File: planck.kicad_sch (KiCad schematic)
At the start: 53 parts, among them J1 USB_C_Receptacle_USB2.0, K1 KEYSW, K2 KEYSW, K3 KEYSW, K4 KEYSW, SW1 SW_PUSH, U1 ATmega32U4-M, Y1 Crystal_GND24_Small

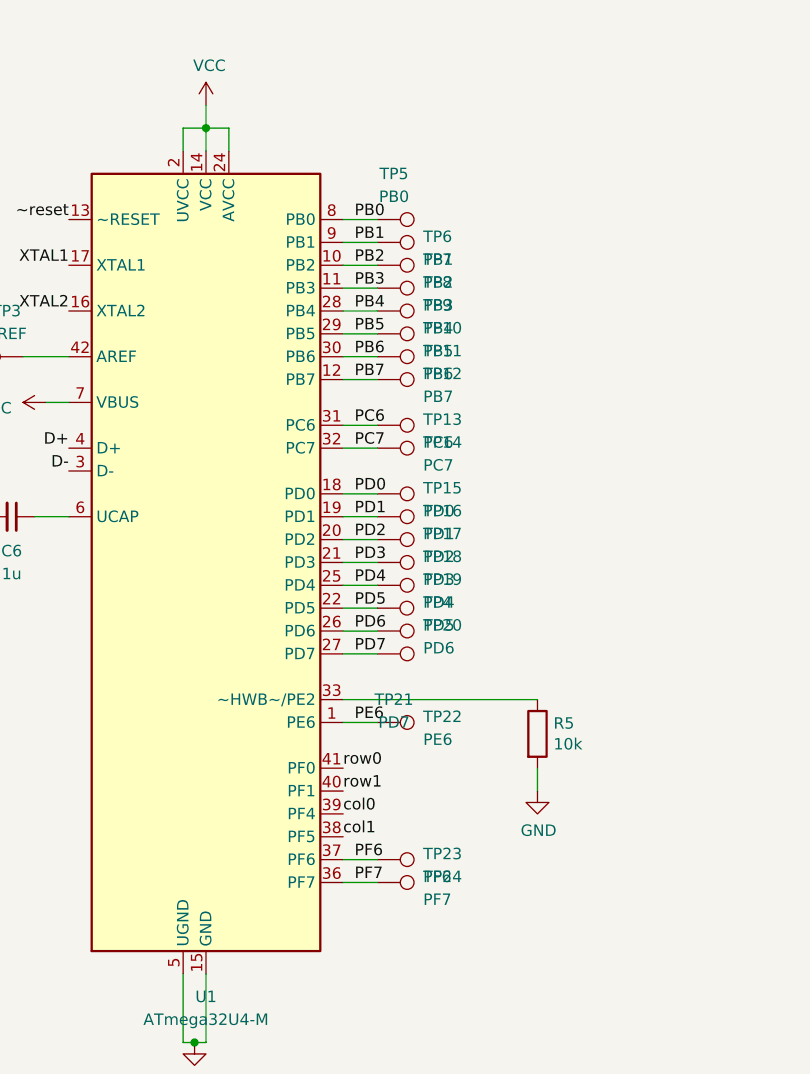
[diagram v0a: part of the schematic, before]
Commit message: finishing it off
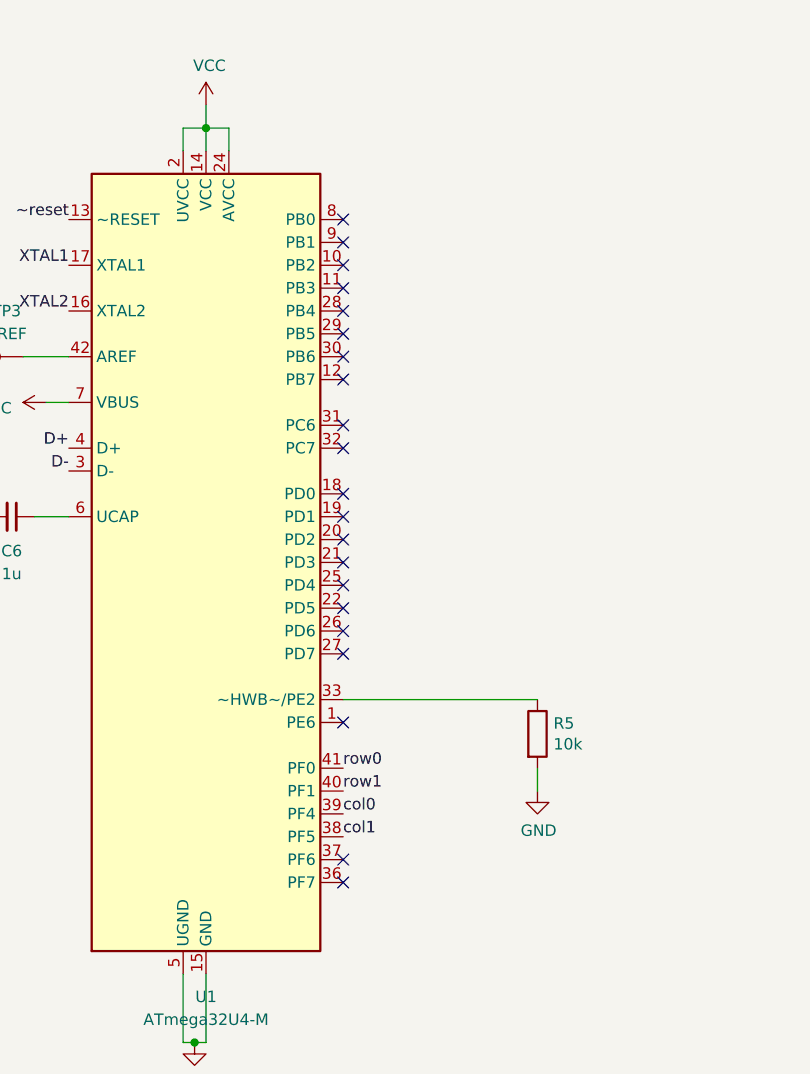
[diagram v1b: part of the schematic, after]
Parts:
- removed TP10: PB5, TestPoint:TestPoint_Pad_D1.0mm, symbol Connector:TestPoint
- removed TP11: PB6, TestPoint:TestPoint_Pad_D1.0mm, symbol Connector:TestPoint
- removed TP12: PB7, TestPoint:TestPoint_Pad_D1.0mm, symbol Connector:TestPoint
- removed TP13: PC6, TestPoint:TestPoint_Pad_D1.0mm, symbol Connector:TestPoint
- removed TP14: PC7, TestPoint:TestPoint_Pad_D1.0mm, symbol Connector:TestPoint
- removed TP15: PD0, TestPoint:TestPoint_Pad_D1.0mm, symbol Connector:TestPoint
- removed TP16: PD1, TestPoint:TestPoint_Pad_D1.0mm, symbol Connector:TestPoint
- removed TP17: PD2, TestPoint:TestPoint_Pad_D1.0mm, symbol Connector:TestPoint
- removed TP18: PD3, TestPoint:TestPoint_Pad_D1.0mm, symbol Connector:TestPoint
- removed TP19: PD4, TestPoint:TestPoint_Pad_D1.0mm, symbol Connector:TestPoint
- removed TP20: PD6, TestPoint:TestPoint_Pad_D1.0mm, symbol Connector:TestPoint
- removed TP21: PD7, TestPoint:TestPoint_Pad_D1.0mm, symbol Connector:TestPoint
- removed TP22: PE6, TestPoint:TestPoint_Pad_D1.0mm, symbol Connector:TestPoint
- removed TP23: PF6, TestPoint:TestPoint_Pad_D1.0mm, symbol Connector:TestPoint
- removed TP24: PF7, TestPoint:TestPoint_Pad_D1.0mm, symbol Connector:TestPoint
- removed TP4: PD5, TestPoint:TestPoint_Pad_D1.0mm, symbol Connector:TestPoint
- removed TP5: PB0, TestPoint:TestPoint_Pad_D1.0mm, symbol Connector:TestPoint
- removed TP6: PB1, TestPoint:TestPoint_Pad_D1.0mm, symbol Connector:TestPoint
- removed TP7: PB2, TestPoint:TestPoint_Pad_D1.0mm, symbol Connector:TestPoint
- removed TP8: PB3, TestPoint:TestPoint_Pad_D1.0mm, symbol Connector:TestPoint
- removed TP9: PB4, TestPoint:TestPoint_Pad_D1.0mm, symbol Connector:TestPoint
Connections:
- net PB0: no longer names the net of U1.8 (PB0)
- net PB1: no longer names the net of U1.9 (PB1)
- net PB2: no longer names the net of U1.10 (PB2)
- net PB3: no longer names the net of U1.11 (PB3)
- net PB4: no longer names the net of U1.28 (PB4)
- net PB5: no longer names the net of U1.29 (PB5)
- net PB6: no longer names the net of U1.30 (PB6)
- net PB7: no longer names the net of U1.12 (PB7)
- net PC6: no longer names the net of U1.31 (PC6)
- net PC7: no longer names the net of U1.32 (PC7)
- net PD0: no longer names the net of U1.18 (PD0)
- net PD1: no longer names the net of U1.19 (PD1)
- net PD2: no longer names the net of U1.20 (PD2)
- net PD3: no longer names the net of U1.21 (PD3)
- net PD4: no longer names the net of U1.25 (PD4)
- net PD5: no longer names the net of U1.22 (PD5)
- net PD6: no longer names the net of U1.26 (PD6)
- net PD7: no longer names the net of U1.27 (PD7)
- net PE6: no longer names the net of U1.1 (PE6)
- net PF6: no longer names the net of U1.37 (PF6)
- net PF7: no longer names the net of U1.36 (PF7)
- no-connect marks 0 -> 21
